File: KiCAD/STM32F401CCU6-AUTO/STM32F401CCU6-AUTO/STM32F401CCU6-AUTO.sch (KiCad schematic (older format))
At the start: 69 parts

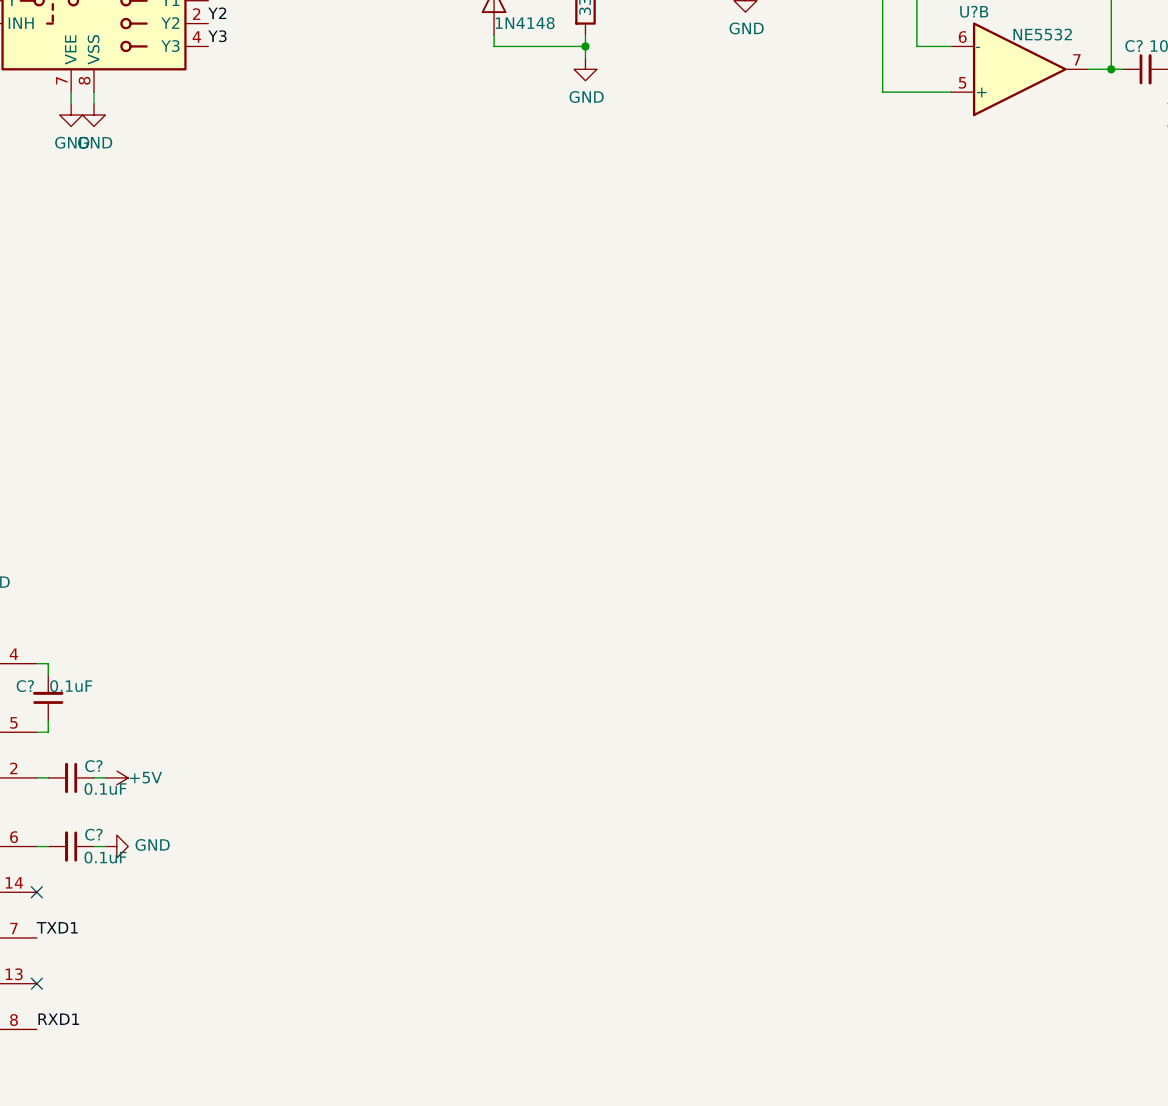
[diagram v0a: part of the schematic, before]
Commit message: add auto
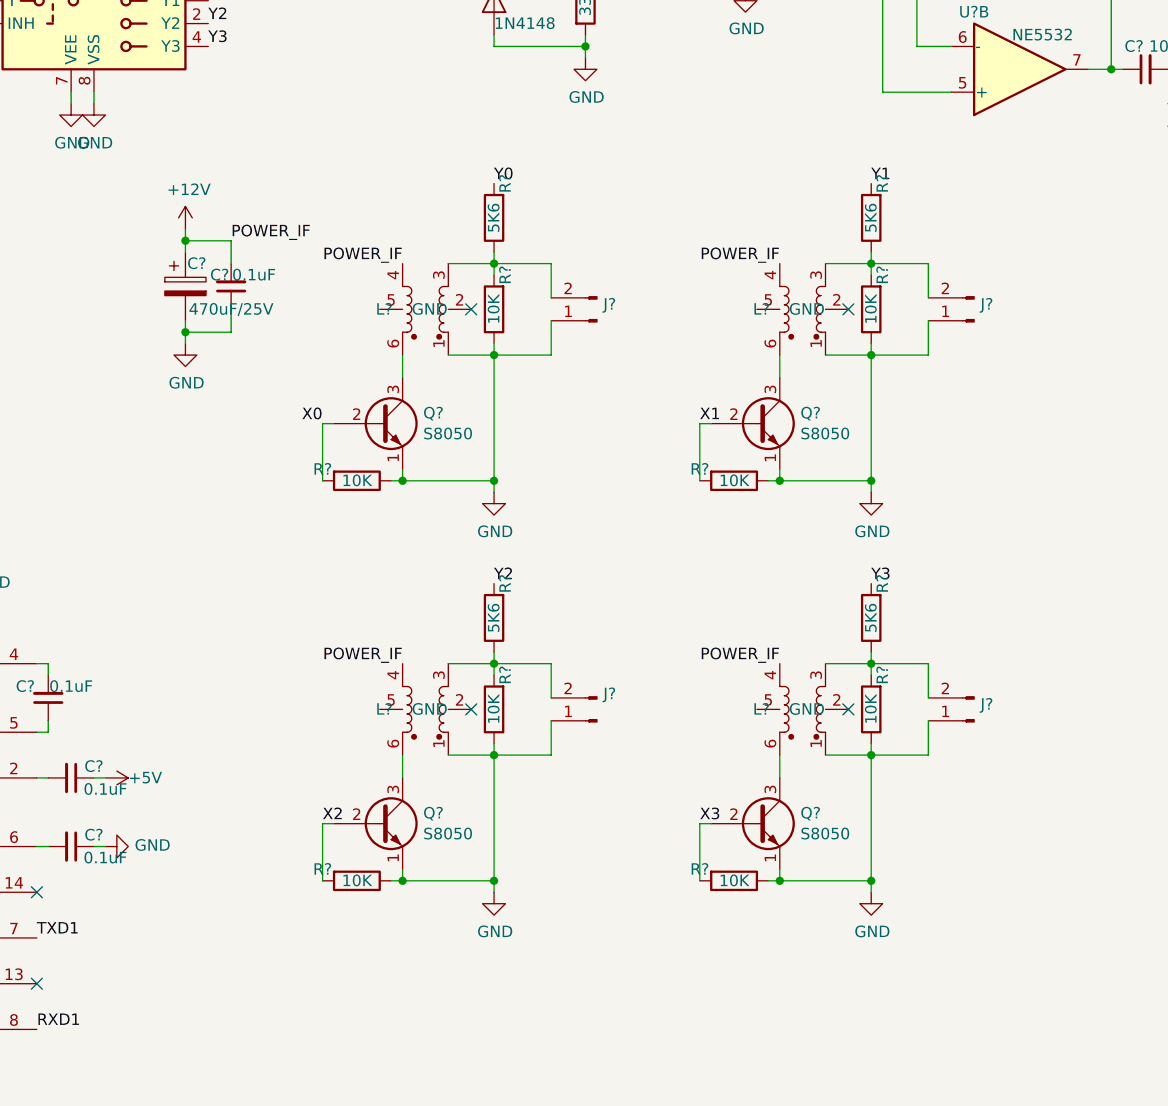
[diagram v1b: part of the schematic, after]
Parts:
- added C?: 470uF/25V, symbol Device:CP
- added C?: 0.1uF, Capacitor_SMD:C_0603_1608Metric_Pad1.05x0.95mm_HandSolder, symbol Device:C_Small
- added J? (x4): Conn_01x02_Male, symbol Connector:Conn_01x02_Male
- added L? (x4): if_amplifier, symbol qmechanics:if_amplifier
- added Q? (x4): S8050, Package_TO_SOT_THT:TO-92_Inline, symbol Transistor_BJT:S8050
- added R? (x8): 10K, Resistor_SMD:R_0402_1005Metric, symbol Device:R
- added R? (x4): 5K6, Resistor_SMD:R_0402_1005Metric, symbol Device:R
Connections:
- net labels added: POWER_IF
- wire segments 234 -> 310
- no-connect marks 20 -> 24
